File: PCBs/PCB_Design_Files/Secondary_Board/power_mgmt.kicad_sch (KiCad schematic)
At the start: 19 parts, among them Q3 MMBT3904, Q4 MMBT3904, U2 MMSZ5221BT1G, U5 TPS61023DRLR, U6 TLV9101IDCKR

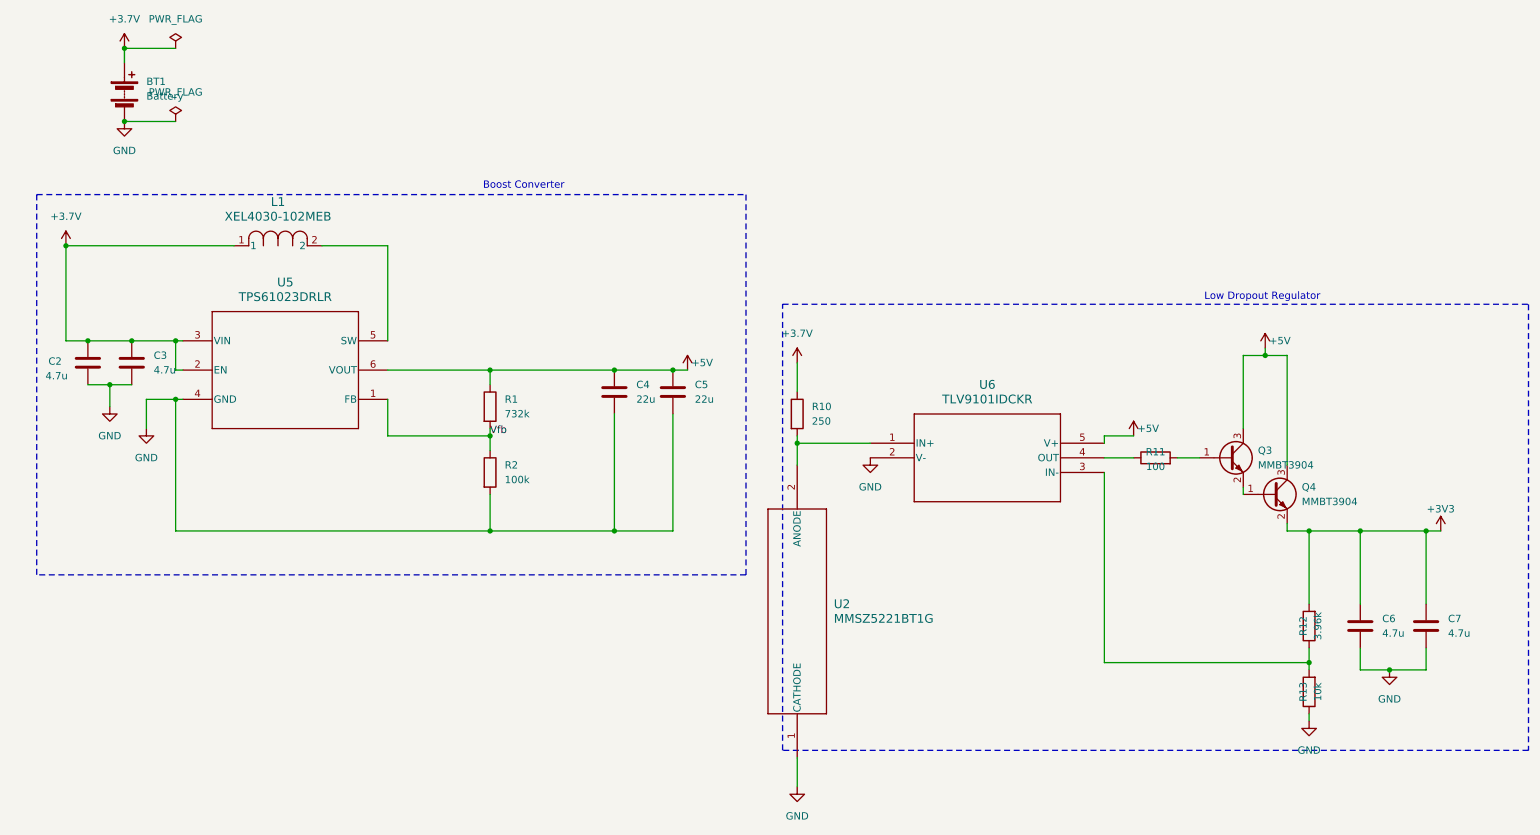
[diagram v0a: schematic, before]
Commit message: secondary board connectors
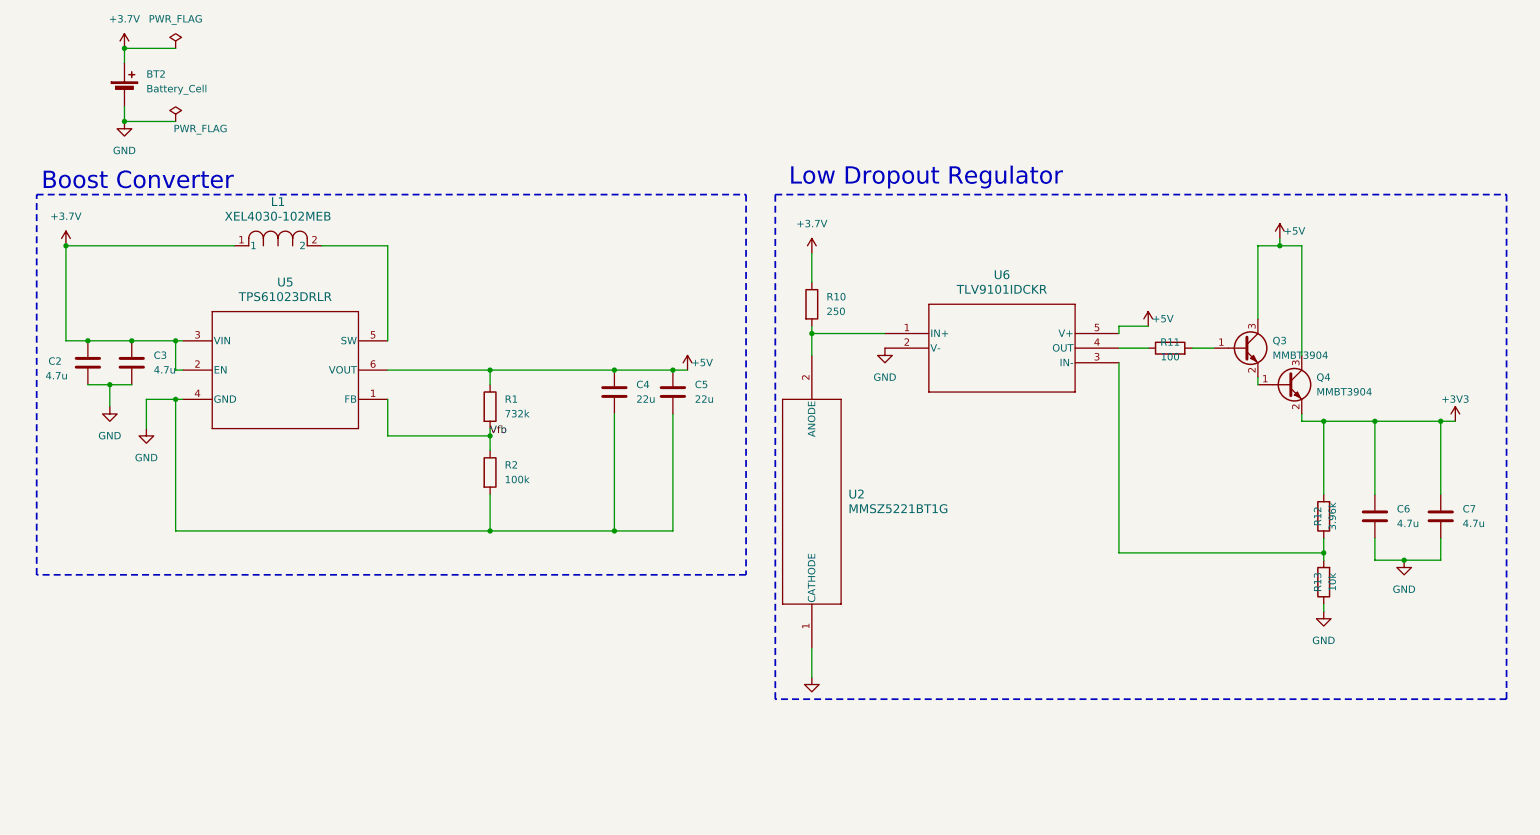
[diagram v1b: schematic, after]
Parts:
- removed BT1: Battery, Connector_JST:JST_PH_S2B-PH-K_1x02_P2.00mm_Horizontal, symbol Device:Battery
- added BT2: Battery_Cell, Project Footprints:bat_pads, symbol Device:Battery_Cell
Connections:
- net +3.7V: now also BT2.1 (+)
- net GND: now also BT2.2 (-)
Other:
- moved on the sheet: C6, C7, Q3, Q4, R10, R11, R12, R13, U2, U6
